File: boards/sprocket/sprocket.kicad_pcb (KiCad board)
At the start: 4 copper layers, 47 x 15 mm, 33 parts, among them J1 SPROCKET-CONN, J4 Conn_01x04_MountingPin, J5 Conn_01x04_MountingPin, J6 Conn_01x04_MountingPin, J7 Conn_01x04_MountingPin, Q1 NX7002BKR, SW1 SW_Push, SW2 SW_Push, U1 STM32G031G8U6, U2 AP2210N-3.3TRG1

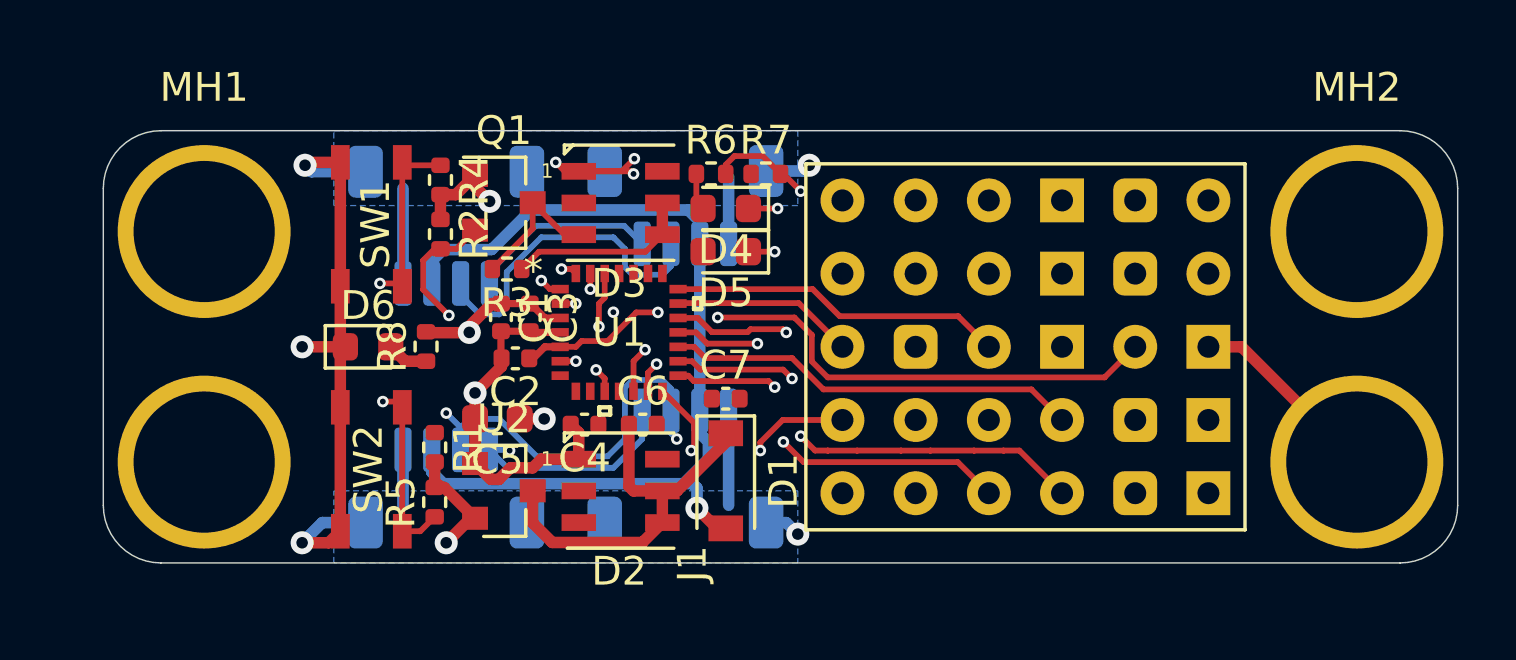
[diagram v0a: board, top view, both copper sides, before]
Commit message: Gunna bail.
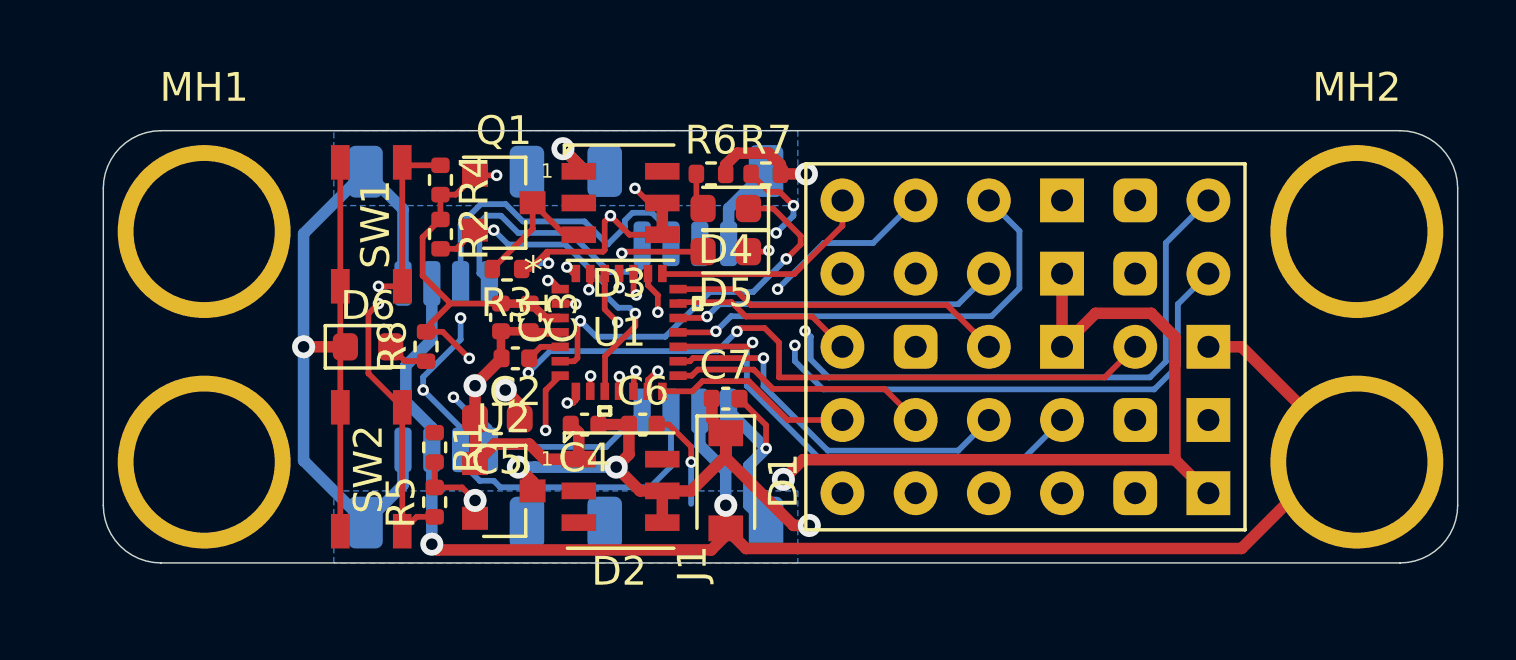
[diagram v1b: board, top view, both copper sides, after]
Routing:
- net +5V: track 31.1 -> 67.0 mm, vias 0 -> 6
- net /UART-TX: track 0.00 -> 32.6 mm, vias 0 -> 2
- net /UART-RX: track 0.00 -> 28.0 mm, vias 0 -> 2
- net +3V3: track 34.5 -> 61.2 mm, vias 5 -> 6
- net /+5v0-RAW: track 39.6 -> 55.3 mm, vias 1 -> 2
- net /SPI-CIPO: track 0.00 -> 13.4 mm, vias 0 -> 2
- net /GPIO1: track 0.00 -> 13.3 mm, vias 0 -> 1
- net /SPI-SCK: track 0.00 -> 13.1 mm, vias 0 -> 1
- net /GPIO2: track 0.00 -> 12.5 mm, vias 0 -> 1
- net GND: track 53.0 -> 64.7 mm, vias 9 -> 5
- net Net-(D5-Pad2): track 0.00 -> 11.6 mm, vias 0 -> 3
- net /SPI-COPI: track 0.00 -> 9.71 mm, vias 0 -> 1
- net /~SPI-CS: track 0.00 -> 7.83 mm
- net /QWIIC2-SCL: track 6.62 -> 9.66 mm
- net /I2C1-SDA: track 33.9 -> 31.3 mm, vias 4 -> 3
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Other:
- board text removed: "TODO: Move buttons to top, LEDs to bottom"

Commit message: About to give up again
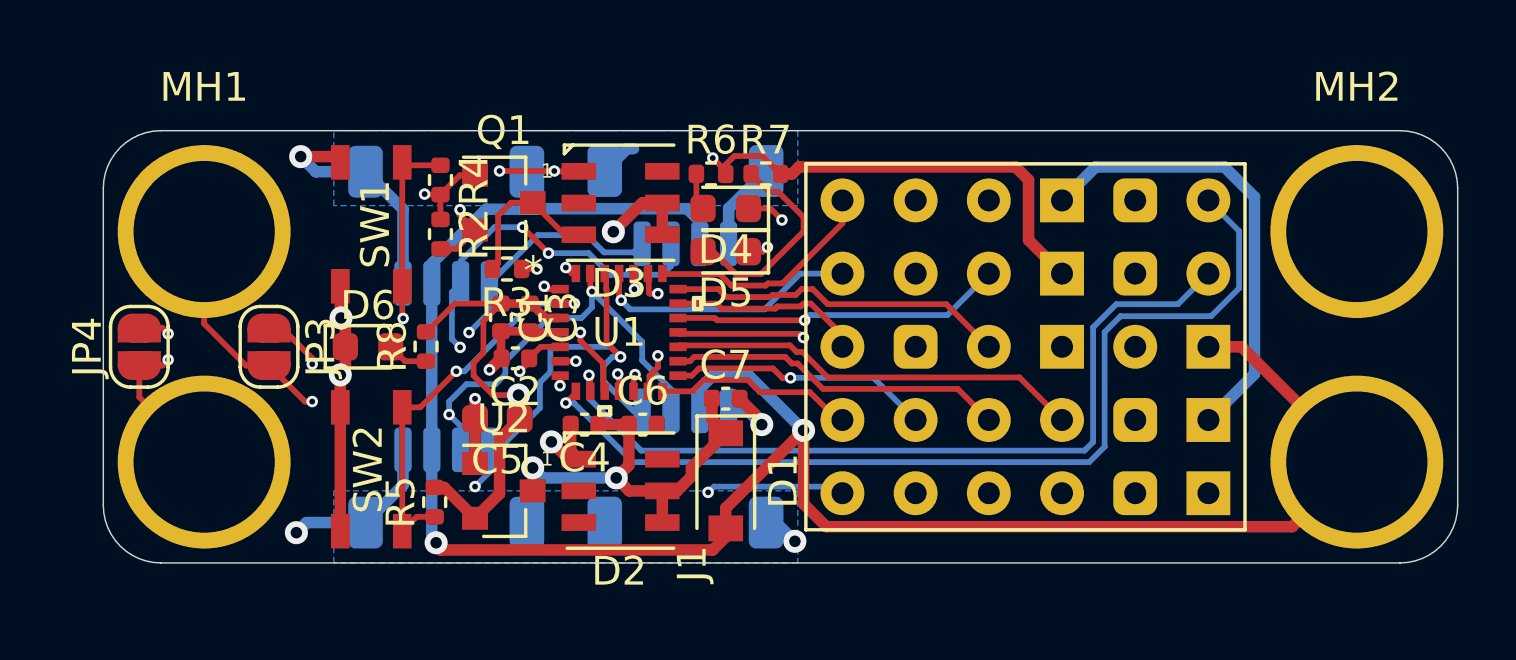
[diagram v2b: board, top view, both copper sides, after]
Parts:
- removed R1: 10K, Resistor_SMD:R_0402_1005Metric
- added JP3: SolderJumper_2_Open, Jumper:SolderJumper-2_P1.3mm_Open_RoundedPad1.0x1.5mm, F.Cu at (106.2, 83.0)
- added JP4: SolderJumper_2_Open, Jumper:SolderJumper-2_P1.3mm_Open_RoundedPad1.0x1.5mm, F.Cu at (101.8, 83.0)
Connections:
- J6 pad 3: /QWIIC2-SDA -> /I2C2-SDA
- J6 pad 4: /QWIIC2-SCL -> /I2C2-SCL
- J7 pad 3: /QWIIC2-SDA -> /I2C2-SDA
- J7 pad 4: /QWIIC2-SCL -> /I2C2-SCL
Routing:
- net /I2C2-SDA: track 11.4 -> 31.6 mm, vias 1 -> 5
- net /I2C2-SCL: track 16.0 -> 33.9 mm, vias 1 -> 3
- net /+5v0-RAW: track 55.3 -> 71.3 mm
- net +3V3: track 61.2 -> 46.5 mm, vias 6 -> 3
- net GND: track 64.7 -> 50.9 mm, vias 5 -> 11
- net +5V: track 67.0 -> 55.2 mm, vias 6 -> 4
- net /QWIIC2-SDA: track 11.5 -> 0.00 mm
- net /QWIIC2-SCL: track 9.66 -> 0.00 mm
- net /I2C1-SCL: track 27.2 -> 32.7 mm, vias 2 -> 3
- net /BUTTON2: track 18.1 -> 13.6 mm
- net Net-(D5-Pad2): track 11.6 -> 7.36 mm, vias 3 -> 0
- net /I2C1-SDA: track 31.3 -> 27.9 mm
- net /SPI-SCK: track 13.1 -> 10.5 mm
- net /GPIO8: track 16.9 -> 14.4 mm, vias 1 -> 0
- net /SPI-CIPO: track 13.4 -> 11.6 mm, vias 2 -> 1
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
